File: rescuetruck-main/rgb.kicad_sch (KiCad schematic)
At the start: 47 parts

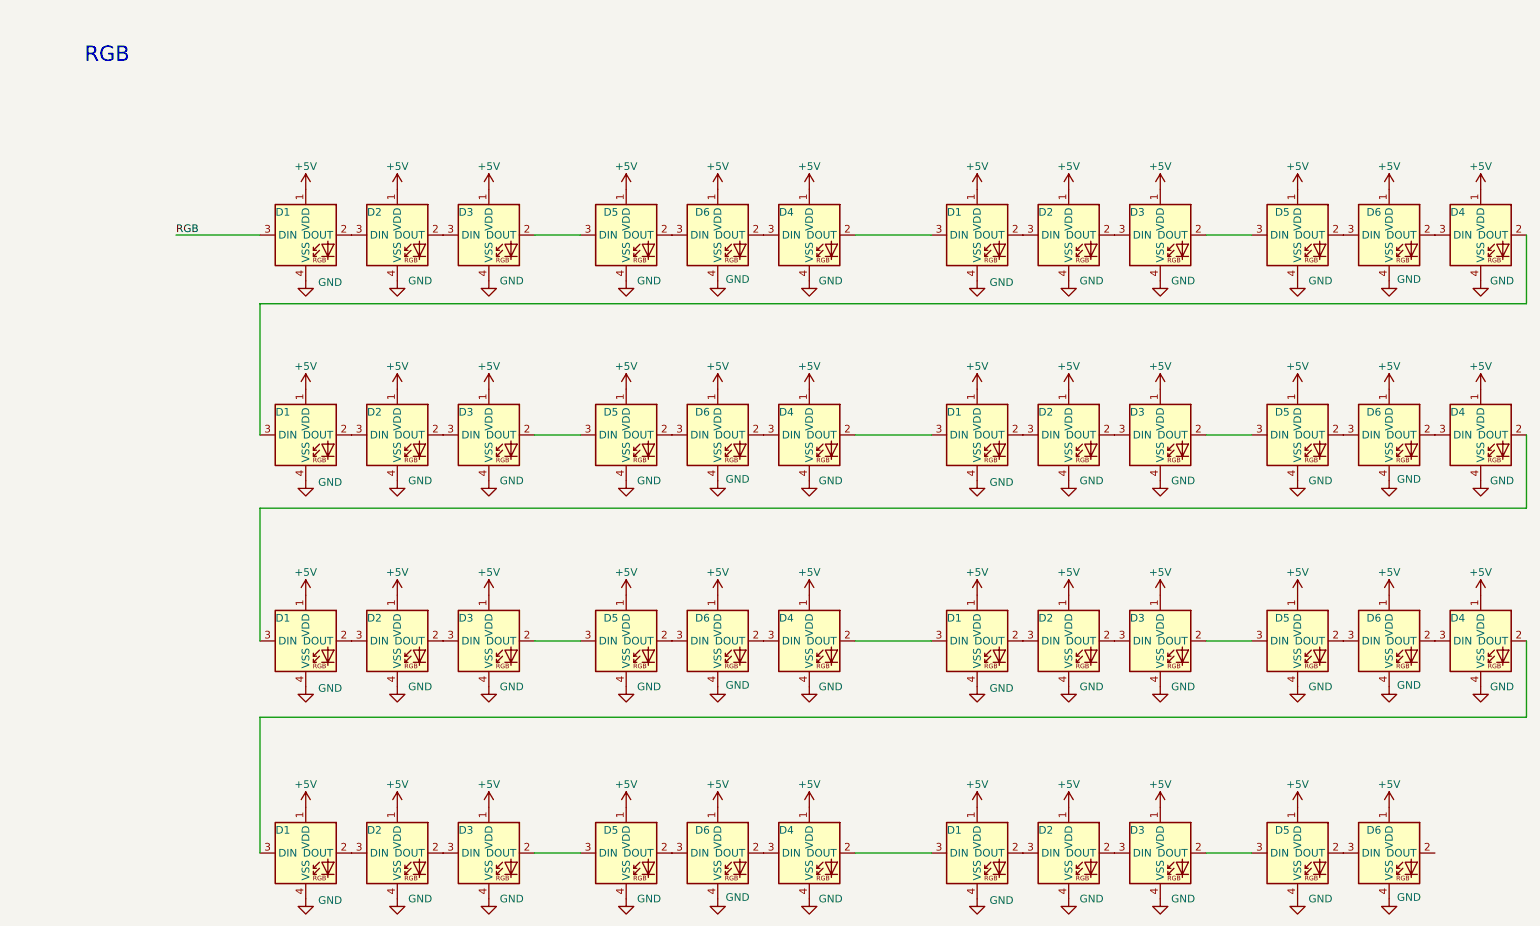
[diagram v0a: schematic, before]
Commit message: vootvan progress
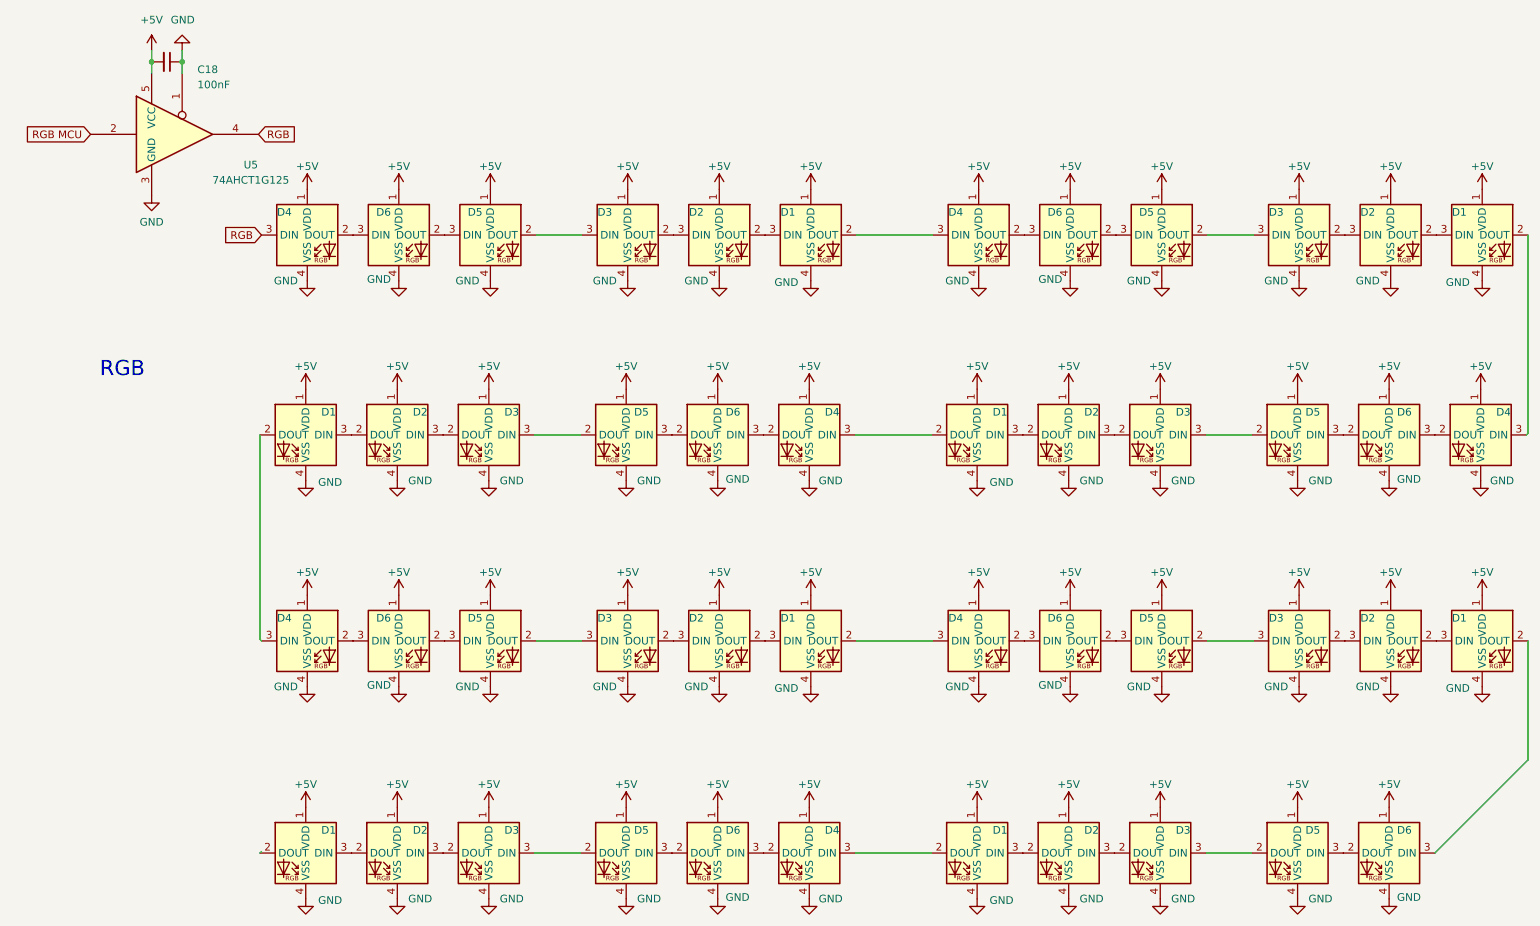
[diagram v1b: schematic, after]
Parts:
- added C18: 100nF, Capacitor_SMD:C_0402_1005Metric, symbol Device:C_Small
- added U5: 74AHCT1G125, Package_TO_SOT_SMD:TSOT-23-5, symbol 74xGxx:74AHCT1G125
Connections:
- net +5V: now also C18.2, U5.5 (VCC)
- net GND: now also C18.1, U5.1, U5.3 (GND)
- net RGB: now also D4.3 (DIN), U5.4; no longer D1.3 (DIN)
- net at D4.2 (DOUT): now also D6.3 (DIN); no longer D1.3 (DIN) (x3)
- net at D4.3 (DIN): now also D1.2 (DOUT); no longer D6.2 (DOUT) (x4)
- net at D3.2 (DOUT): now also D2.3 (DIN); no longer D5.3 (DIN) (x3)
- net at D3.3 (DIN): now also D5.2 (DOUT); no longer D2.2 (DOUT) (x3)
- net at D5.2 (DOUT): now also D3.3 (DIN); no longer D6.3 (DIN) (x4)
- net at D5.3 (DIN): now also D6.2 (DOUT); no longer D3.2 (DOUT) (x4)
- net at D1.2 (DOUT): now also D6.3 (DIN); no longer D2.3 (DIN)
- net at D6.3 (DIN): now also D4.2 (DOUT); no longer D5.2 (DOUT) (x3)
- net at D6.2 (DOUT): now also D5.3 (DIN); no longer D4.3 (DIN) (x3)
- net at D2.2 (DOUT): now also D1.3 (DIN); no longer D3.3 (DIN) (x5)
- net at D2.3 (DIN): now also D3.2 (DOUT); no longer D1.2 (DOUT) (x4)
- net at D1.2 (DOUT): now also D4.3 (DIN); no longer D2.3 (DIN) (x2)
- net at D1.3 (DIN): now also D2.2 (DOUT); no longer D4.2 (DOUT) (x3)
- net at D1.2 (DOUT): no longer D2.3 (DIN)
- net at D6.2 (DOUT): now also D5.3 (DIN)
- new net: D2.3 (DIN), D3.2 (DOUT)
- new net: D4.2 (DOUT), D6.3 (DIN)
- new net: D3.3 (DIN), D5.2 (DOUT)
- new net RGB MCU: U5.2
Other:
- moved on the sheet: D1, D2, D3, D4, D5, D6
